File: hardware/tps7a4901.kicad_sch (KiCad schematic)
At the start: 8 parts, among them U3 TPS7A4901DGNR

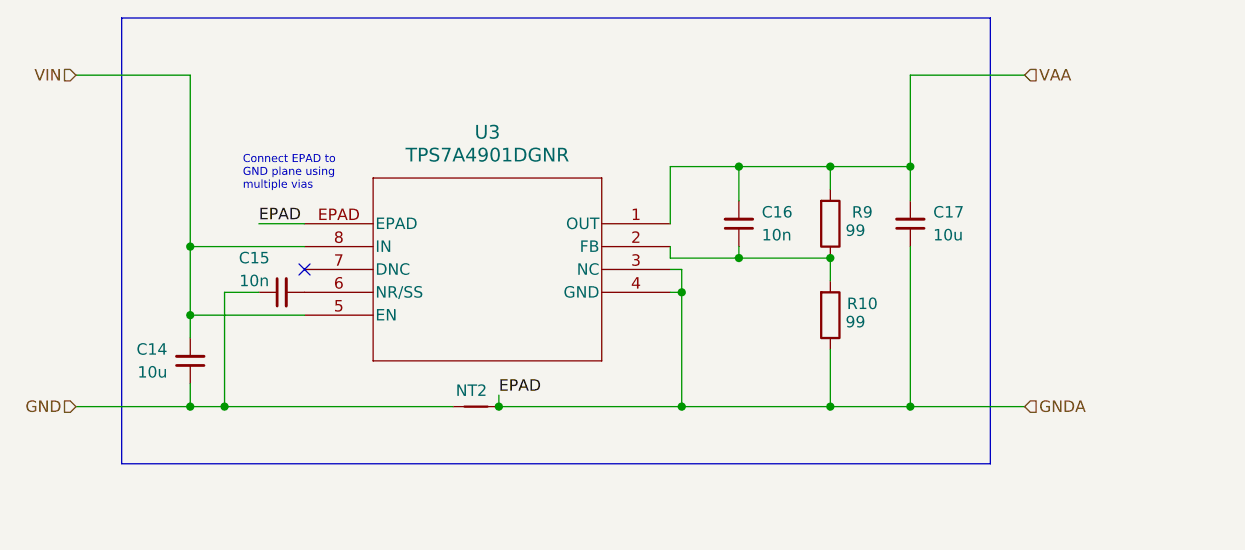
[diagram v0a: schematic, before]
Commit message: minor tweaks
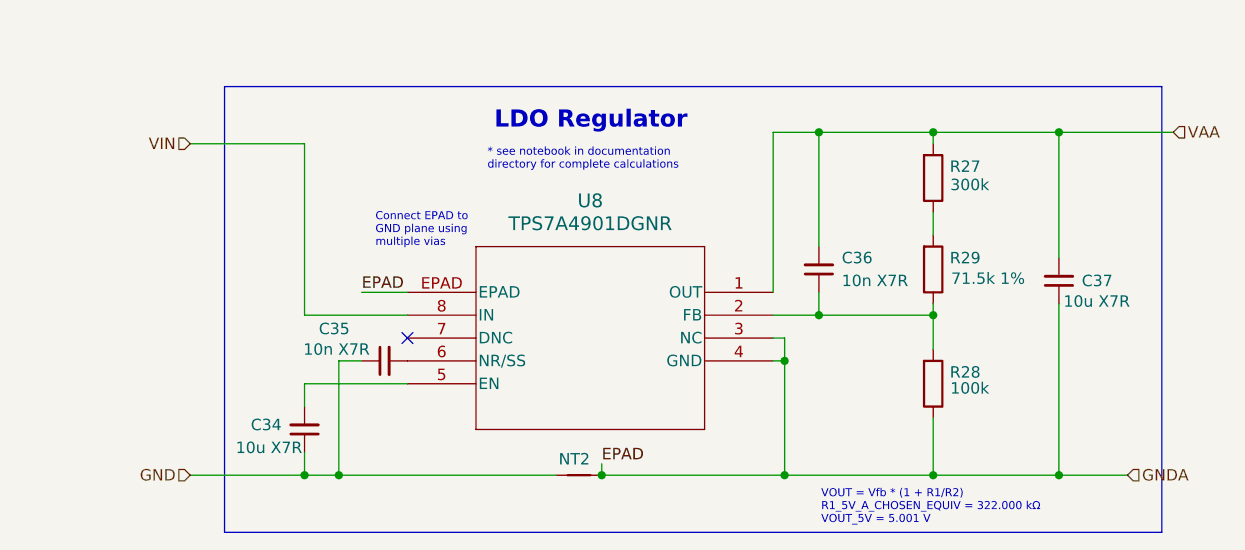
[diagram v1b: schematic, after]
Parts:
- removed C14, C17: 10u, Capacitor_SMD:C_0805_2012Metric_Pad1.18x1.45mm_HandSolder, symbol Device:C_Small
- removed C15, C16: 10n, Capacitor_SMD:C_0805_2012Metric_Pad1.18x1.45mm_HandSolder, symbol Device:C_Small
- removed R10, R9: 99, Resistor_SMD:R_0805_2012Metric_Pad1.20x1.40mm_HandSolder, symbol Device:R
- removed U3: TPS7A4901DGNR, kml-custom:DGN8_1P89X1P57, symbol kml-custom:TPS7A4901DGNR
- added C34, C37: 10u X7R, Capacitor_SMD:C_1206_3216Metric, symbol Device:C_Small
- added C35, C36: 10n X7R, Capacitor_SMD:C_1206_3216Metric, symbol Device:C_Small
- added R27: 300k, symbol Device:R
- added R28: 100k, symbol Device:R
- added R29: 71.5k 1%, symbol Device:R
- added U8: TPS7A4901DGNR, kml-custom:DGN8_1P89X1P57, symbol kml-custom:TPS7A4901DGNR
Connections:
- net GND: now also C34.1, C35.1
- net GNDA: now also C37.1, R28.1, U8.3 (NC), U8.4 (GND), U8.EPAD
- net VAA: now also C36.2, C37.2, R27.2, U8.1 (OUT)
- net VIN: now also U8.8 (IN)
- new net: C34.2, U8.5 (EN)
- new net: C36.1, R28.2, R29.1, U8.2 (FB)
- new net: C35.2, U8.6 (NR/SS)
- new net: R27.1, R29.2
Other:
- note added: "* see notebook in documentation directory for complete calculations"
- note added: "LDO Regulator"
- note added: "VOUT = Vfb * (1 + R1/R2) R1_5V_A_CHOSEN_EQUIV = 322.000 kΩ VOUT_5V = 5.001 V"
